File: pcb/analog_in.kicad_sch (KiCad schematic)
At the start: 8 parts

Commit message: Updated footprints
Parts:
- Abstandssensor_1: footprint Connector:FanPinHeader_1x04_P2.54mm_Vertical -> Connector_Phoenix_MSTB:PhoenixContact_MSTBA_2,5_4-G-5,08_1x04_P5.08mm_Horizontal
- Anemometer_1: footprint (none) -> Connector_Phoenix_MSTB:PhoenixContact_MSTBA_2,5_8-G-5,08_1x08_P5.08mm_Horizontal
- Kraftsensor_1: footprint (none) -> Connector_Phoenix_MSTB:PhoenixContact_MSTBA_2,5_4-G-5,08_1x04_P5.08mm_Horizontal
- R1: footprint Resistor_SMD:R_0201_0603Metric -> Resistor_SMD:R_1206_3216Metric
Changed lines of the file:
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@@
       (effects (font (size 1.27 1.27)) (justify left))
     )
-    (property "Footprint" "Resistor_SMD:R_0201_0603Metric" (at 59.182 109.22 90)
+    (property "Footprint" "Resistor_SMD:R_1206_3216Metric" (at 59.182 109.22 90)
       (effects (font (size 1.27 1.27)) hide)
     )
@@
       (effects (font (size 1.27 1.27)))
     )
-    (property "Footprint" "" (at 21.59 59.69 0)
+    (property "Footprint" "Connector_Phoenix_MSTB:PhoenixContact_MSTBA_2,5_4-G-5,08_1x04_P5.08mm_Horizontal" (at 21.59 59.69 0)
       (effects (font (size 1.27 1.27)) hide)
     )
@@
       (effects (font (size 1.27 1.27)))
     )
-    (property "Footprint" "" (at 21.59 101.6 0)
+    (property "Footprint" "Connector_Phoenix_MSTB:PhoenixContact_MSTBA_2,5_8-G-5,08_1x08_P5.08mm_Horizontal" (at 21.59 101.6 0)
       (effects (font (size 1.27 1.27)) hide)
     )
@@
       (effects (font (size 1.27 1.27)) (justify left))
     )
-    (property "Footprint" "Resistor_SMD:R_0201_0603Metric" (at 50.292 63.5 90)
+    (property "Footprint" "Resistor_SMD:R_1206_3216Metric" (at 50.292 63.5 90)
       (effects (font (size 1.27 1.27)) hide)
     )
@@
       (effects (font (size 1.27 1.27)) (justify left))
     )
-    (property "Footprint" "Resistor_SMD:R_0201_0603Metric" (at 36.322 33.02 90)
+    (property "Footprint" "Resistor_SMD:R_1206_3216Metric" (at 36.322 33.02 90)
       (effects (font (size 1.27 1.27)) hide)
     )
@@
       (effects (font (size 1.27 1.27)) (justify left))
     )
-    (property "Footprint" "Resistor_SMD:R_0201_0603Metric" (at 50.292 73.66 90)
+    (property "Footprint" "Resistor_SMD:R_1206_3216Metric" (at 50.292 73.66 90)
       (effects (font (size 1.27 1.27)) hide)
     )
@@
       (effects (font (size 1.27 1.27)))
     )
-    (property "Footprint" "Connector:FanPinHeader_1x04_P2.54mm_Vertical" (at 21.59 24.13 0)
+    (property "Footprint" "Connector_Phoenix_MSTB:PhoenixContact_MSTBA_2,5_4-G-5,08_1x04_P5.08mm_Horizontal" (at 21.59 24.13 0)
       (effects (font (size 1.27 1.27)) hide)
     )
@@
       (effects (font (size 1.27 1.27)) (justify left))
     )
-    (property "Footprint" "Resistor_SMD:R_0201_0603Metric" (at 51.562 109.22 90)
-      (effects (font (size 1.27 1.27)) hide)
-    )
+    (property "Footprint" "Resistor_SMD:R_1206_3216Metric" (at 51.562 109.22 90)
+      (effects (font (size 1.27 1.27)) hide)
+    )

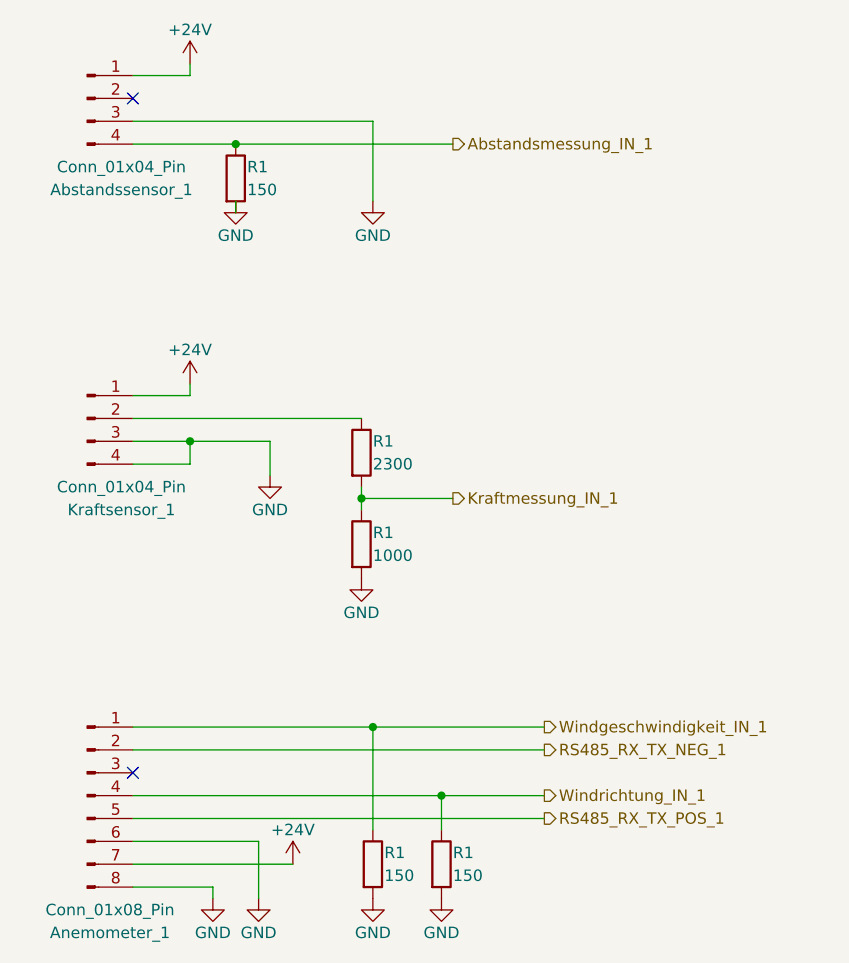
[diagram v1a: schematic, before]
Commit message: updated pcb
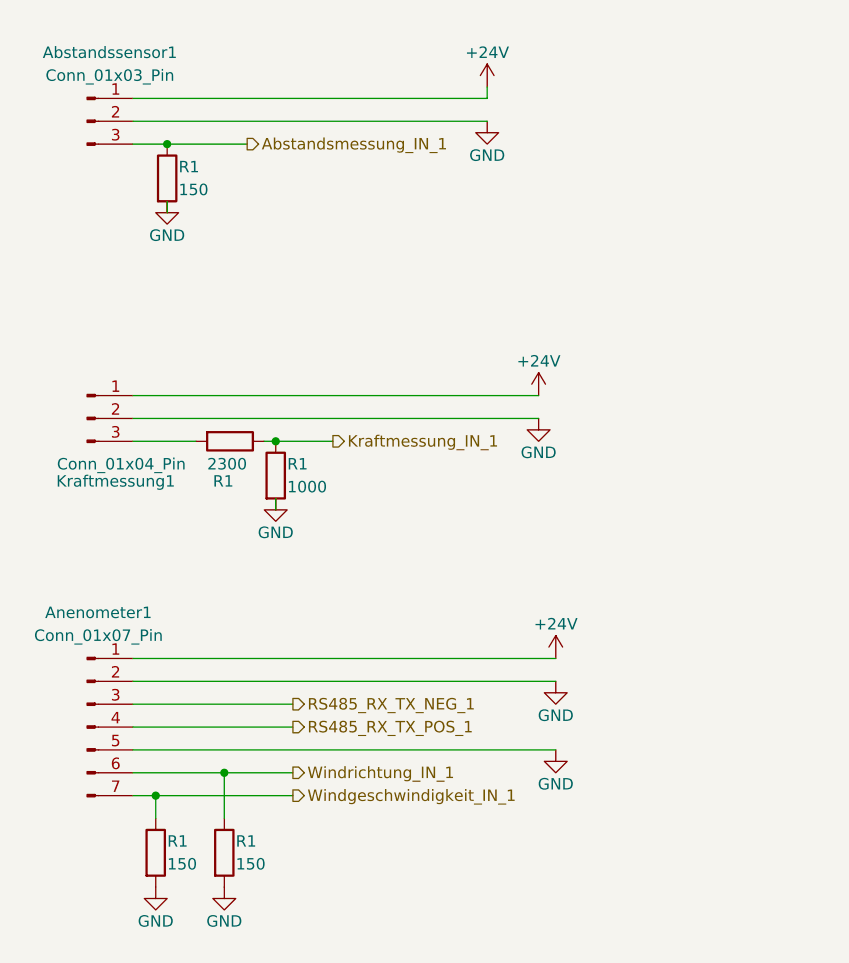
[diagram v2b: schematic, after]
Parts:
- removed Abstandssensor_1: Conn_01x04_Pin, Connector_Phoenix_MSTB:PhoenixContact_MSTBA_2,5_4-G-5,08_1x04_P5.08mm_Horizontal, symbol Connector:Conn_01x04_Pin
- removed Anemometer_1: Conn_01x08_Pin, Connector_Phoenix_MSTB:PhoenixContact_MSTBA_2,5_8-G-5,08_1x08_P5.08mm_Horizontal, symbol Connector:Conn_01x08_Pin
- removed R1: 2300, Resistor_SMD:R_1206_3216Metric, symbol Device:R
- removed R1: 1000, Resistor_SMD:R_1206_3216Metric, symbol Device:R
- added Abstandssensor1: Conn_01x03_Pin, TerminalBlock_TE-Connectivity:TerminalBlock_TE_282834-3_1x03_P2.54mm_Horizontal, symbol Connector:Conn_01x03_Pin
- added Anenometer1: Conn_01x07_Pin, TerminalBlock_TE-Connectivity:TerminalBlock_TE_282834-7_1x07_P2.54mm_Horizontal, symbol Connector:Conn_01x07_Pin
- added R1: 1000, Resistor_SMD:R_1206_3216Metric, symbol Device:R
- added R1: 2300, Resistor_SMD:R_1206_3216Metric, symbol Device:R
- Kraftmessung1: renamed from Kraftsensor_1; footprint Connector_Phoenix_MSTB:PhoenixContact_MSTBA_2,5_4-G-5,08_1x04_P5.08mm_Horizontal -> TerminalBlock_TE-Connectivity:TerminalBlock_TE_282834-3_1x03_P2.54mm_Horizontal; symbol Connector:Conn_01x04_Pin -> Connector:Conn_01x03_Pin
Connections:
- net +24V: now also Abstandssensor1.1 (Pin_1), Anenometer1.1 (Pin_1)
- net Abstandsmessung_IN_1: now also Abstandssensor1.3 (Pin_3)
- net GND: now also Kraftmessung1.2 (Pin_2), Abstandssensor1.2 (Pin_2), Anenometer1.2 (Pin_2), Anenometer1.5 (Pin_5), R1.2; no longer Kraftmessung1.3 (Pin_3), Kraftmessung1.4 (Pin_4)
- net Kraftmessung_IN_1: now also R1.1, R1.1
- net RS485_RX_TX_NEG_1: now also Anenometer1.3 (Pin_3)
- net RS485_RX_TX_POS_1: now also Anenometer1.4 (Pin_4)
- net Windgeschwindigkeit_IN_1: now also Anenometer1.7 (Pin_7)
- net Windrichtung_IN_1: now also Anenometer1.6 (Pin_6)
- new net: Kraftmessung1.3 (Pin_3), R1.2
- no-connect marks 2 -> 0
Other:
- moved on the sheet: R1
